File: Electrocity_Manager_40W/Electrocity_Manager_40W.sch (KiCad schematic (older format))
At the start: 197 parts, among them IC2 MAIN_SHUTDOWN, IC3 RELAY_STATE, IC4 ADC_RST, J1 SERIAL, P1 SWD, P10 EMERGENCY, P11 EMERGENCY, P12 FRAME_GRAND, P13 BATT_IN, P15 OUT_B, P16 BATT_IN, P17 OUT_A, P2 CAN, P3 CAN, P4 EMERGENCY_SIGNAL, P5 EMERGENCY_SIGNAL, P6 12V_OUT, P7 12V_OUT, P9 MAIN_SW, Q1 FET_N, Q2 NPN, Q3 NPN, Q4 FET_N, Q7 FET_N, SW1 RST, SW2 SW0, SW3 SW1, U1 MAX3051, U10 BD9G101G, U11 OUTA_CHECK, U12 LOGO, U13 LOGO, U14 OUTB_CHECK, U15 BD33FA1, U16 LOGO, U17 LOGO, U18 LOGO, U19 MCP2221A, U2 STM32F405RG, U20 OSRB38C9AA, U21 OSRB38C9AA, U22 HSIN_946, U23 LOGO, U25 LOGO, U3 FULL COLOR, U4 AQM0802_BL, U5 AP3211, U6 SI8900, U7 AZ1086H, U8 ACS70331, U9 LOGO, X1 8MHz

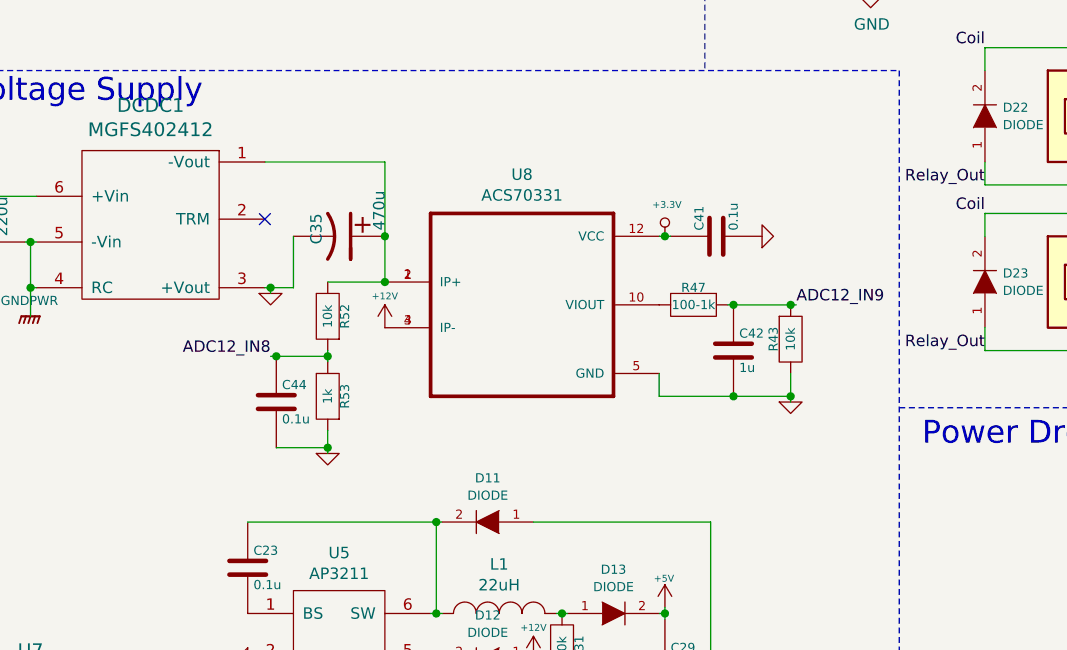
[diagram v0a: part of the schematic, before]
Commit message: normal MD構成大体固まった
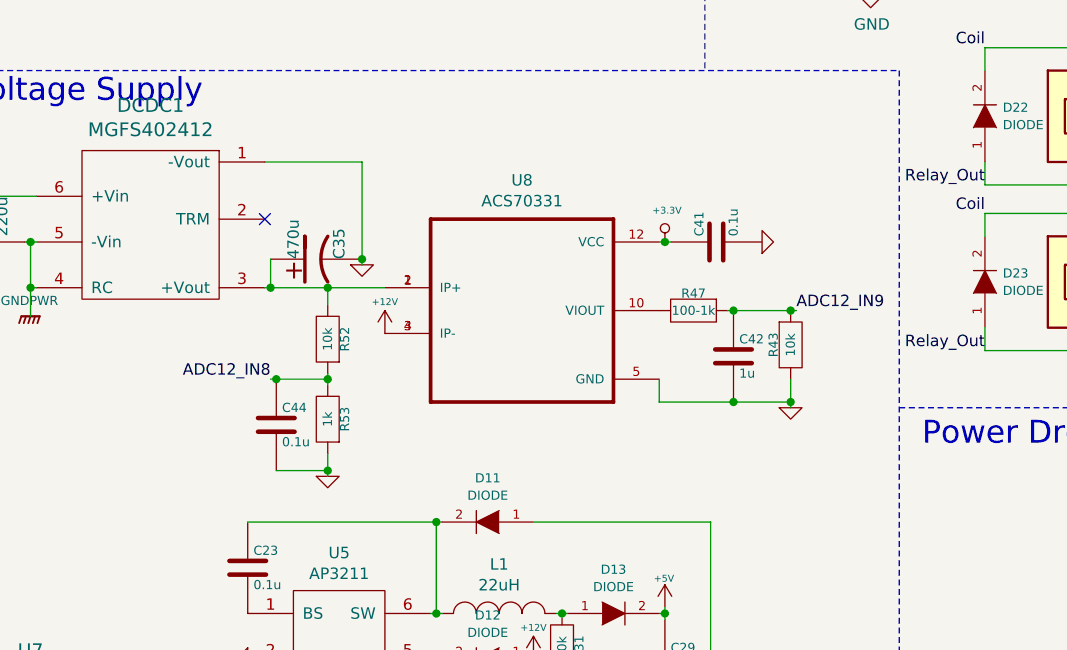
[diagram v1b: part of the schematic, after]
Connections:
- net GND: now also DCDC1.1 (-Vout); no longer DCDC1.3 (+Vout)
- net at C35.1, R52.2, U8.1 (IP+)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: now also DCDC1.3 (+Vout); no longer DCDC1.1 (-Vout)
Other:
- moved on the sheet: C35, C41, C42, C44, R43, R47, R52, R53, U8
